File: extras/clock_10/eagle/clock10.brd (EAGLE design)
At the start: 91 x 96 mm, 120 parts, among them IC101 DC-DC-STEP-DOWN-LM2596, IC102 DS3231W, IC103 1117 3V3, IC104 ZOPT2201, IC105 BME280, IC106 74AC245DW, IC107 74AC245DW, IC201 ESP32S2, IC202 ESP12F, IC203 ESP32C3-MODULE13U, IC204 ESP12F, IC301 1117 3V3, IC302 BME280, J101 12V, J102 IN, J104 4P-2.0, J105 4P-2.0, J201 USB_1, J202 COM, J203 COM, J204 COM, J205 COM, J206 USB_2, J207 OUT_2, J208 OUT_1, J209 OUT_3, J301 IN, SW101 PRG, SW102 RST, U101 SI7021, U301 SI7021, X101 +5V, X102 SHT22, X103 AM2320, X301 +5V, X302 DHT22, X303 AM2320

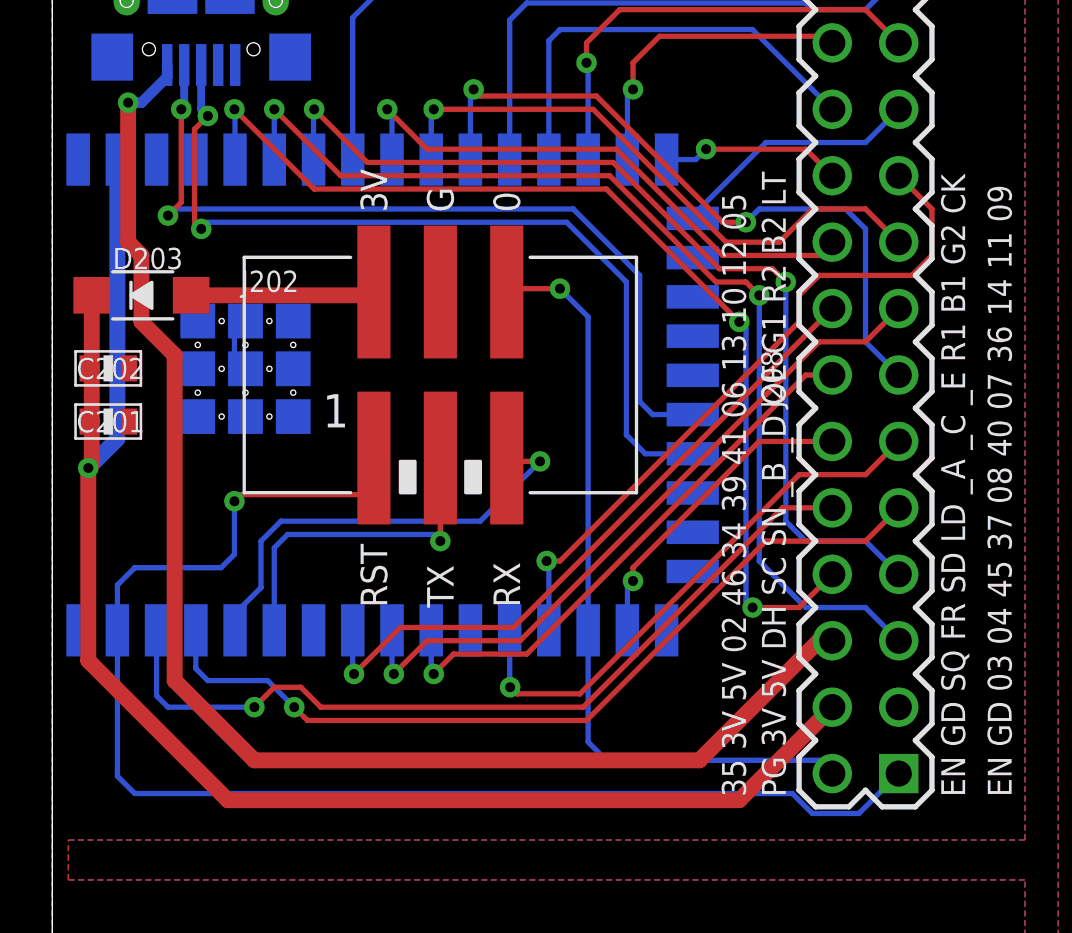
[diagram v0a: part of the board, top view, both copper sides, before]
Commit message: add s2
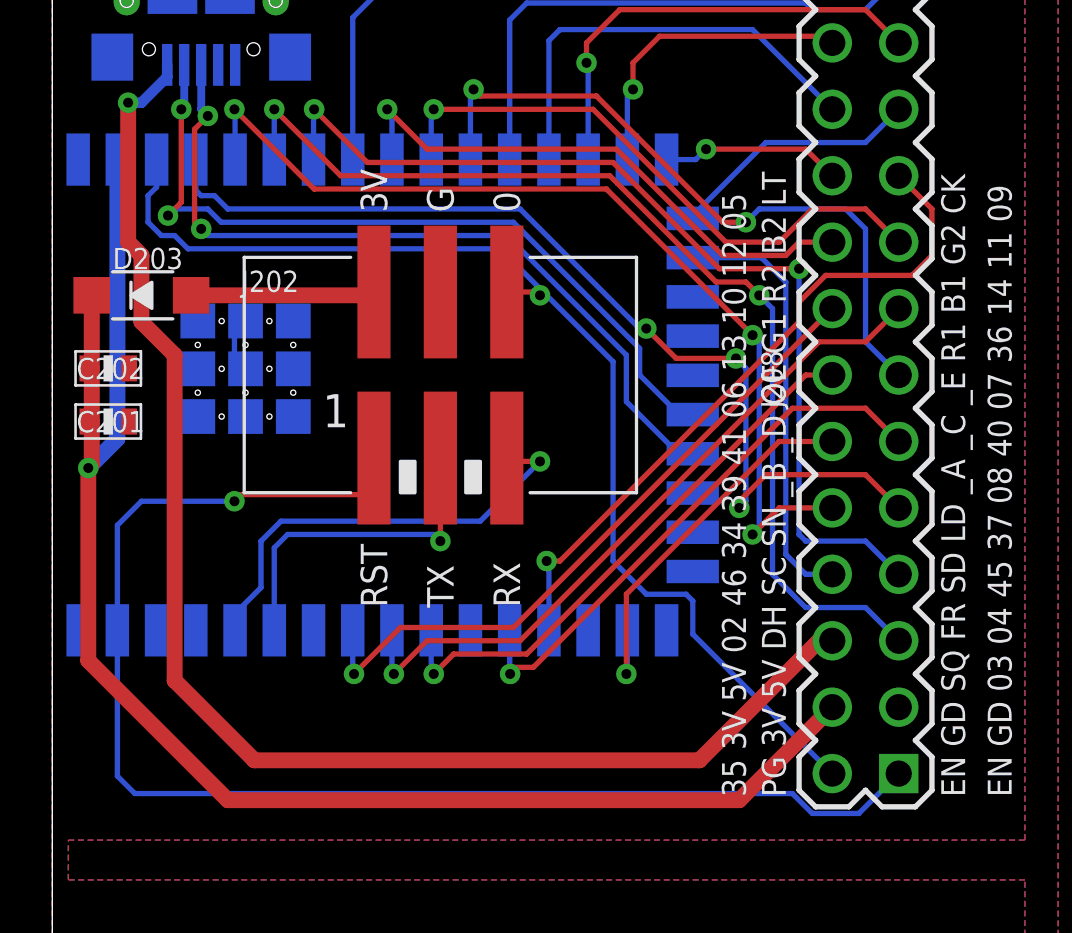
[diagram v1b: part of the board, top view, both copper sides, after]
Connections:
- net I33 renamed 1IO33
- net IO16 renamed 1IO16
- net IO17 renamed 1IO17
- net IO18 renamed 1IO18
- net IO21 renamed 1IO21
- net IO26 renamed 1IO26
- net IO38 renamed 1IO38
- net IO42 renamed 1IO42
- removed net IO15: IC201.I15
- new net 1IO15: IC201.I15, J208.8
- net 1IO0: now also J202.6, J208.2
- net 1IO1: now also J208.9
- net 1IO2: now also J208.10; no longer J208.8
- net 1IO35: no longer J202.6, J208.2
- net 1IO45: no longer J208.9
- net 1IO46: no longer J208.10
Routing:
- net 1IO0: track 0.00 -> 44.2 mm, vias 0 -> 1
- net 1IO1: track 0.00 -> 37.8 mm, vias 0 -> 3
- net 1IO45: track 32.5 -> 0.00 mm, vias 1 -> 0
- net 1IO46: track 32.3 -> 0.00 mm, vias 1 -> 0
- net 1IO35: track 29.7 -> 0.00 mm, vias 1 -> 0
- net 1IO15: track 0.00 -> 16.5 mm
- net 1IO34: track 12.1 -> 15.0 mm
- net 1IO2: track 39.3 -> 36.6 mm
- net 1IO20: track 32.7 -> 30.1 mm
- net 1IO19: track 32.3 -> 30.0 mm
- net 1IO4: track 37.0 -> 37.6 mm
